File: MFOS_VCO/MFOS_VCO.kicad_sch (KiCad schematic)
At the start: 73 parts, among them J1 Conn_02x05_Odd_Even, J10 Jack-DC, J11 Jack-DC, J12 Conn_01x01, J13 Conn_01x01, J14 Conn_01x01, J15 Conn_01x01, J16 Conn_01x01, J17 Conn_01x01, J18 Conn_01x01, J19 Conn_01x01, J2 Jack-DC, J20 Jack-DC, J21 Conn_01x01, J22 Conn_01x01, J23 Conn_01x01, J24 Conn_01x03, J25 Conn_01x01, J26 Conn_01x03, J3 Jack-DC, J4 Jack-DC, J5 Jack-DC, J6 Jack-DC, J7 Jack-DC, J8 Jack-DC, J9 Jack-DC, Q1 PN4391, U1 OP275, U2 TL072, U3 SSM2212, U4 TL074, U5 LM13700, U6 TL072

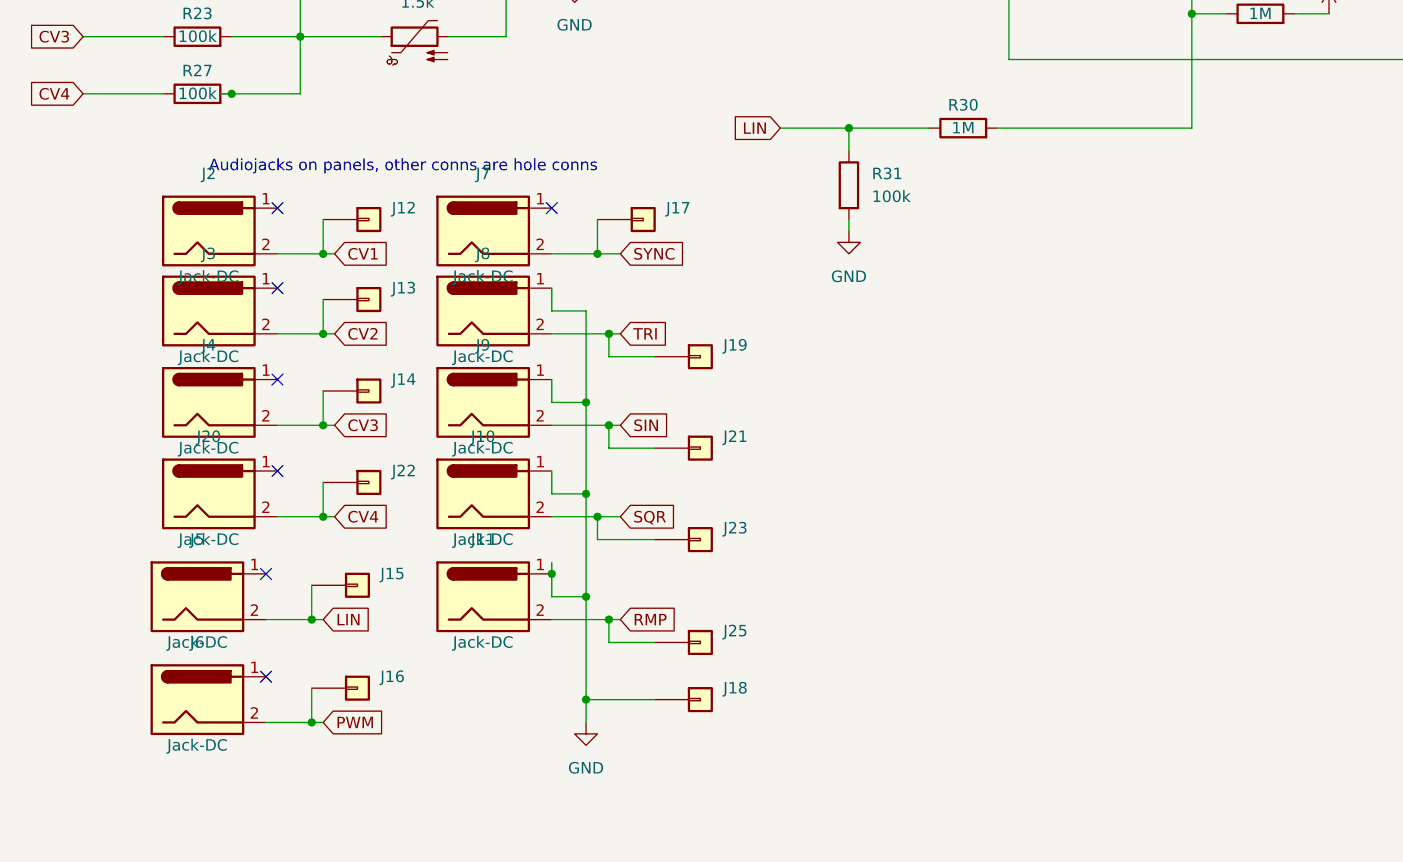
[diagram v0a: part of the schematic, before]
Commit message: Laying out
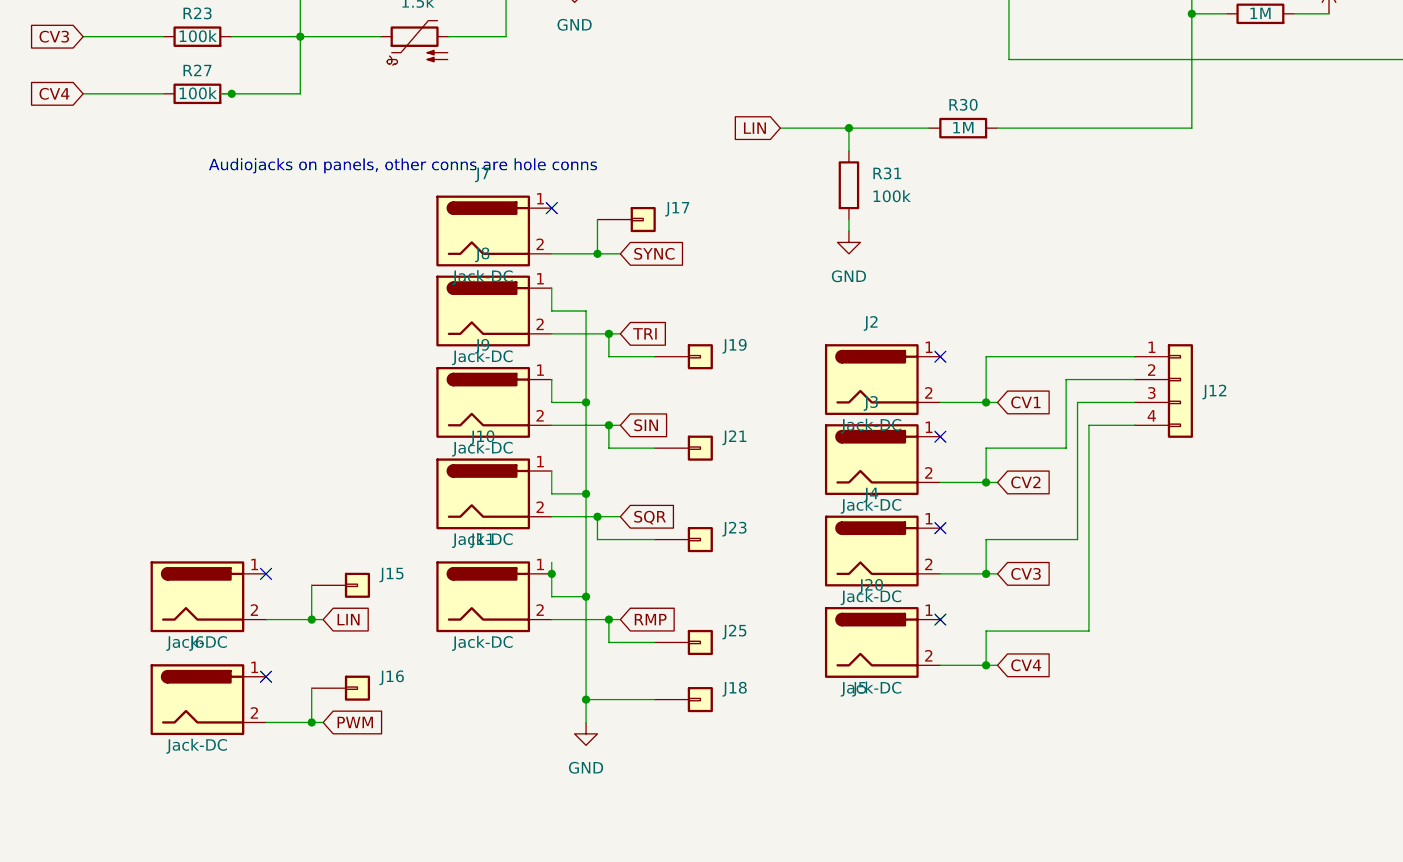
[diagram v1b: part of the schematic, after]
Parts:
- removed J12, J13, J14, J22: Conn_01x01, Connector_Pin:Pin_D1.0mm_L10.0mm_LooseFit, symbol Connector_Generic:Conn_01x01
- added J12: Conn_01x04, Connector_PinHeader_2.54mm:PinHeader_1x04_P2.54mm_Vertical, symbol Connector_Generic:Conn_01x04
- R11, R16: footprint Resistor_THT:R_Axial_DIN0207_L6.3mm_D2.5mm_P7.62mm_Horizontal -> Potentiometer_THT:Potentiometer_Bourns_3339P_Vertical
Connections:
- net CV1: now also J12.1 (Pin_1)
- net CV2: now also J12.2 (Pin_2)
- net CV3: now also J12.3 (Pin_3)
- net CV4: now also J12.4 (Pin_4)
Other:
- moved on the sheet: J2, J20, J3, J4
